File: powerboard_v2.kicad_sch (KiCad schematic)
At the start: 26 parts, among them J1 Conn_01x02_Pin, J2 Conn_01x02_Pin, J3 Conn_01x02_Pin, J7 Conn_01x04_Socket, J8 Conn_ST_STDC14, SW1 SW_Wuerth_450301014042, SW2 SW_Push, U1 STM32F303K8Tx, U2 BD33FC0FP, U3 MCP2562-E-P, U4 BD50FC0FP

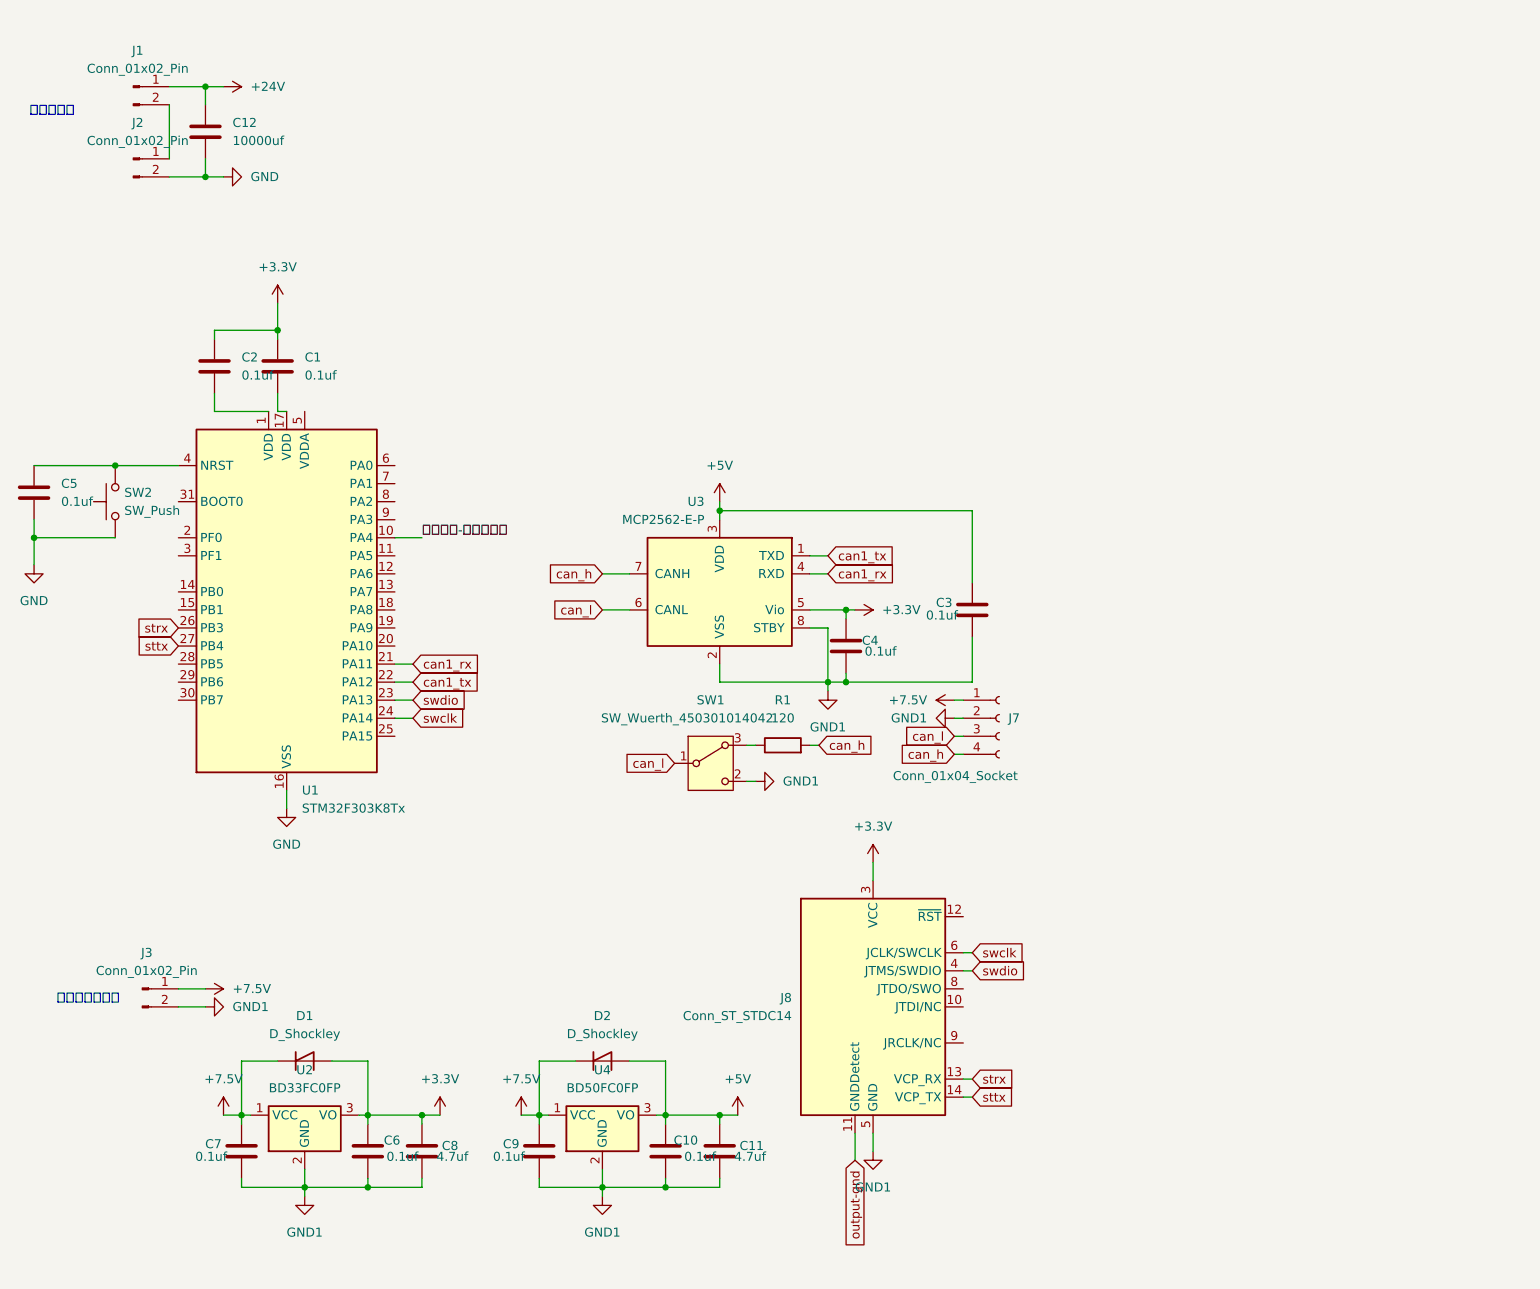
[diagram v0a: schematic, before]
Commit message: 一応バックアップ
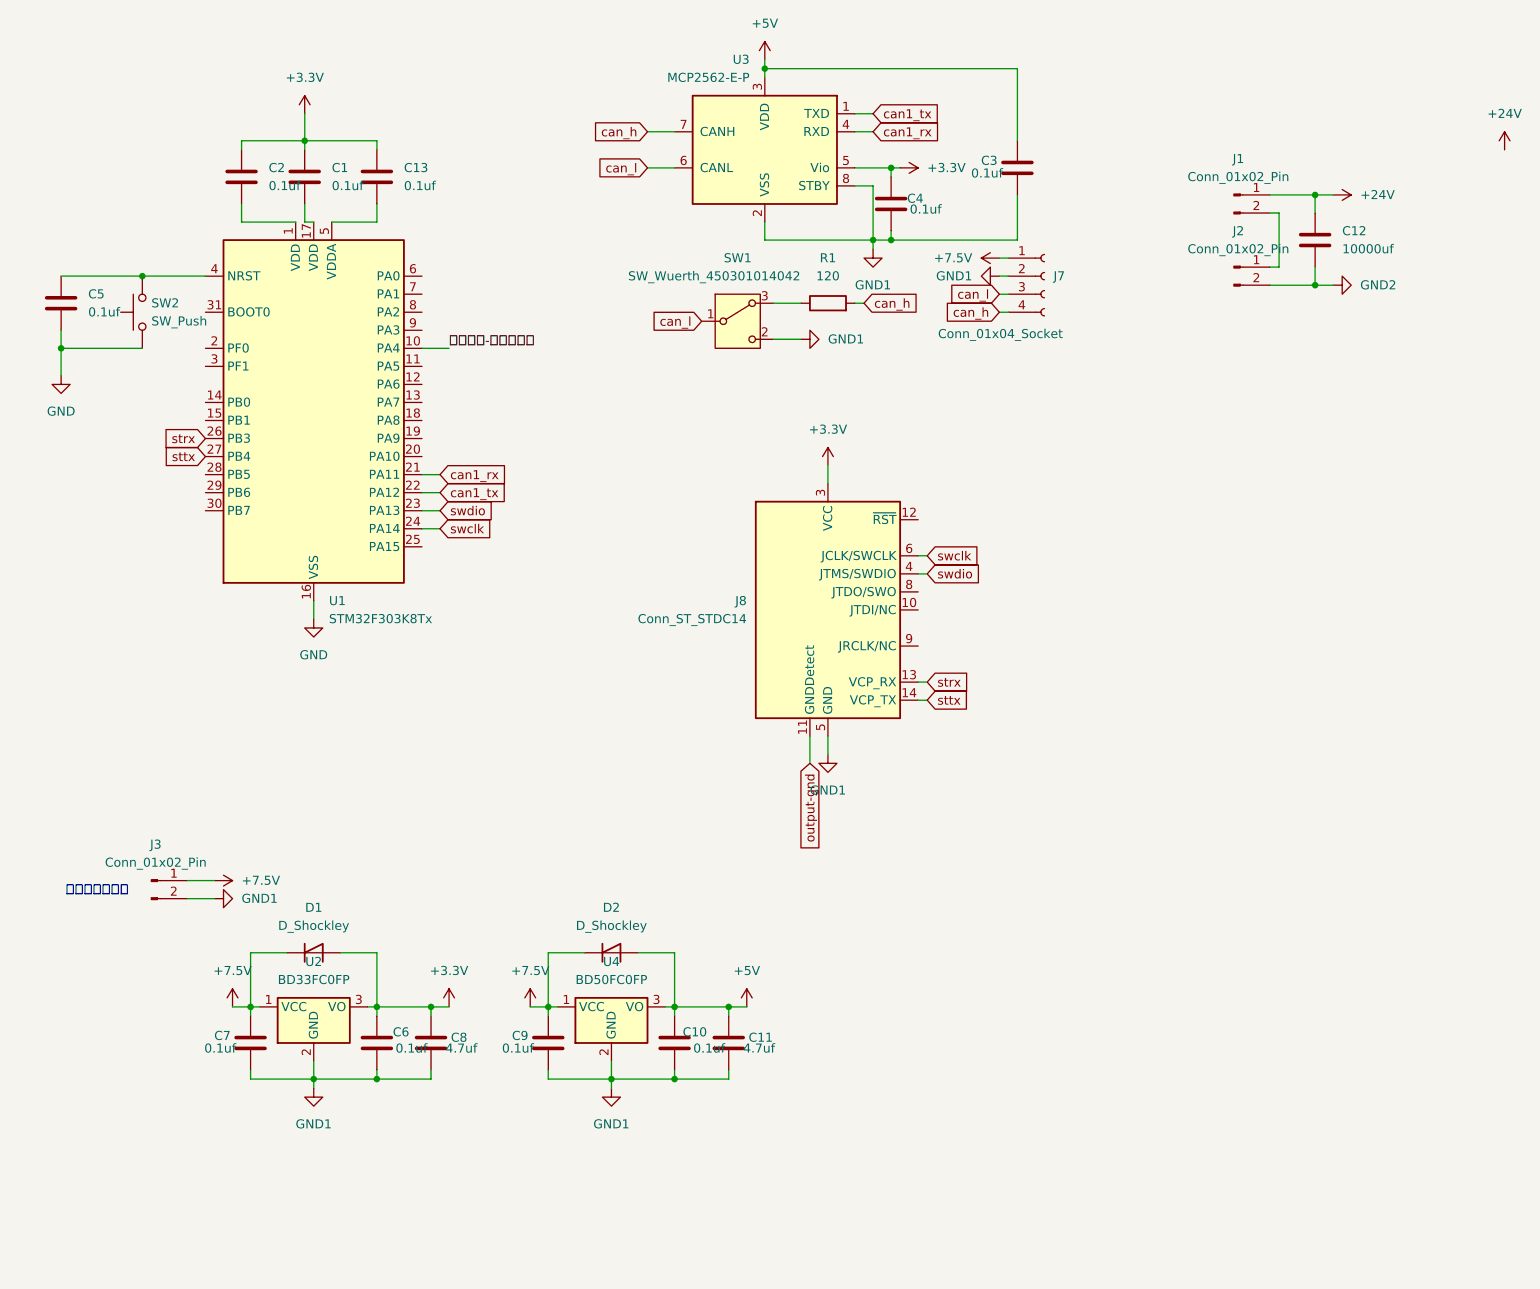
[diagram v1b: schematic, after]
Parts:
- added C13: 0.1uf, symbol Device:C
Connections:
- net +3.3V: now also C13.1
- net GND: no longer C12.2, J2.2 (Pin_2)
- net at U1.5 (VDDA): now also C13.2
- new net GND2: C12.2, J2.2 (Pin_2)
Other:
- note removed: "駆動用電源"
- moved on the sheet: C1, C10, C11, C2, C3, C4, C5, C6, C7, C8, C9, D1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
